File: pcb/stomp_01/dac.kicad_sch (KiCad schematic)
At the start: 20 parts, among them J12 Headphones, U4 AP7313-18SAG, U5 SGTL5000XNLA3

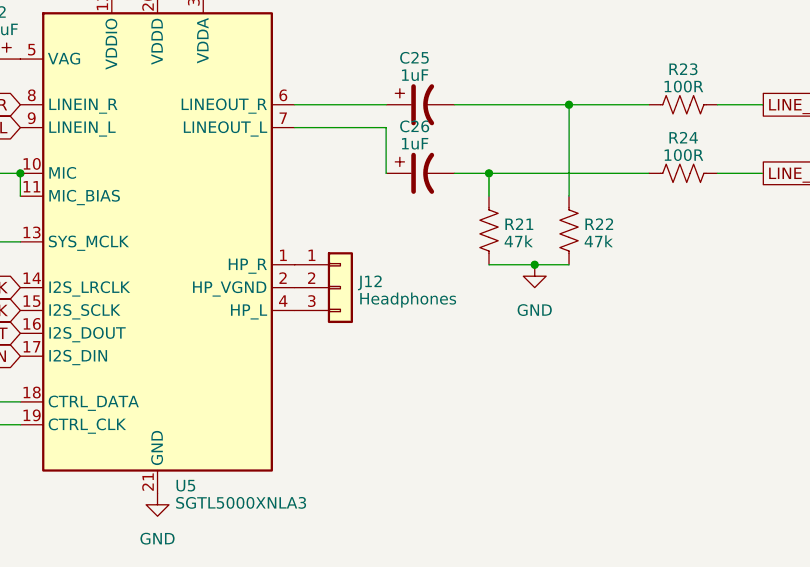
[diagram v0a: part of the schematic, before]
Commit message: pre routing
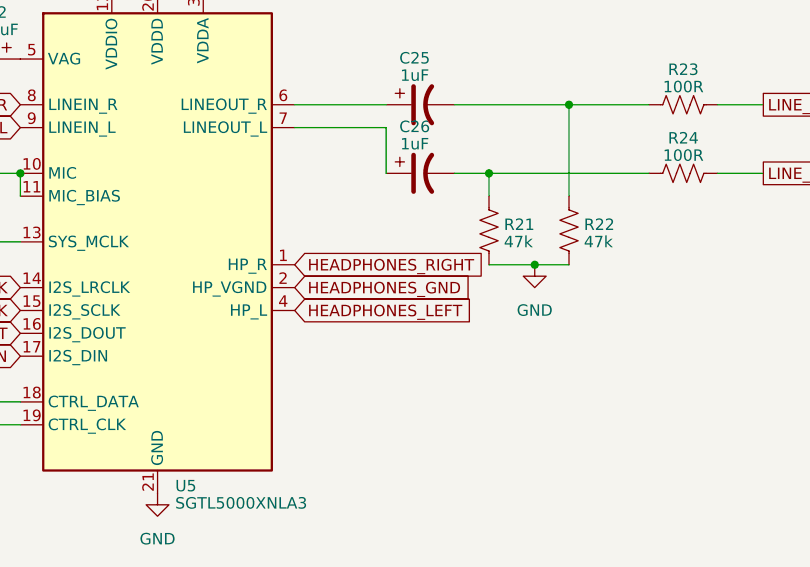
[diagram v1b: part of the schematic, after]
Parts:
- removed J12: Headphones, Connector_PinHeader_2.54mm:PinHeader_1x03_P2.54mm_Vertical, symbol Connector_Generic:Conn_01x03
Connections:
- net HEADPHONES_RIGHT: now reaches U5.1 (HP_R)
- net HEADPHONES_GND: now reaches U5.2 (HP_VGND)
- net HEADPHONES_LEFT: now reaches U5.4 (HP_L)
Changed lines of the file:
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@@
+		)
+	)
+	(global_label "HEADPHONES_LEFT"
+		(shape input)
+		(at 158.75 104.14 0)
+		(fields_autoplaced yes)
+		(effects
+			(font
+				(size 1.27 1.27)
+			)
+			(justify left)
+		)
+		(property "Intersheetrefs" "${INTERSHEET_REFS}"
+			(at 179.3942 104.14 0)
+			(effects
+				(font
+					(size 1.27 1.27)
+				)
+				(justify left)
+				(hide yes)
+			)
+		)
+	)
+	(global_label "HEADPHONES_GND"
+		(shape input)
+		(at 158.75 101.6 0)
+		(fields_autoplaced yes)
+		(effects
+			(font
+				(size 1.27 1.27)
+			)
+			(justify left)
+		)
+		(property "Intersheetrefs" "${INTERSHEET_REFS}"
+			(at 179.0314 101.6 0)
+			(effects
+				(font
+					(size 1.27 1.27)
+				)
+				(justify left)
+				(hide yes)
+			)
+		)
+	)
+	(global_label "HEADPHONES_RIGHT"
+		(shape input)
+		(at 158.75 99.06 0)
+		(fields_autoplaced yes)
+		(effects
+			(font
+				(size 1.27 1.27)
+			)
+			(justify left)
+		)
+		(property "Intersheetrefs" "${INTERSHEET_REFS}"
+			(at 180.6038 99.06 0)
+			(effects
+				(font
+					(size 1.27 1.27)
+				)
+				(justify left)
+				(hide yes)
+			)
 		)
 	)
@@
 					(unit 1)
 				)
-			)
-		)
-	)
-	(symbol
-		(lib_id "Connector_Generic:Conn_01x03")
-		(at 163.83 101.6 0)
-		(unit 1)
-		(exclude_from_sim no)
-		(in_bom yes)
-		(on_board yes)
-		(dnp no)
-		(fields_autoplaced yes)
-		(property "Reference" "J12"
-			(at 165.862 100.9563 0)
-			(effects
-				(font
-					(size 1.27 1.27)
-				)
-				(justify left)
-			)
-		)
-		(property "Value" "Headphones"
-			(at 165.862 102.8773 0)
-			(effects
-				(font
-					(size 1.27 1.27)
-				)
-				(justify left)
-			)
-		)
-		(property "Footprint" "Connector_PinHeader_2.54mm:PinHeader_1x03_P2.54mm_Vertical"
-			(at 163.83 101.6 0)
-			(effects
-				(font
-					(size 1.27 1.27)
-				)
-				(hide yes)
-			)
-		)
-		(property "Datasheet" "~"
-			(at 163.83 101.6 0)
-			(effects
-				(font
-					(size 1.27 1.27)
-				)
-				(hide yes)
-			)
-		)
-		(property "Description" ""
-			(at 163.83 101.6 0)
-			(effects
-				(font
-					(size 1.27 1.27)
-				)
-			)
-		)
-		(pin "1"
-		)
-		(pin "2"
-		)
-		(pin "3"
-		)
-		(instances
-			(project "stomp_00"
-				(path "/8f4a2eb0-078b-46cb-b534-a4acd11d130e/7598c0f0-0137-4b50-80b5-b929d25c284a"
-					(reference "J12")
-					(unit 1)
-				)
